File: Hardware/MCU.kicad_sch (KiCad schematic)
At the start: 23 parts, among them U1 STM32F407VET6, U3 LAN8742A, Y1 25MHz

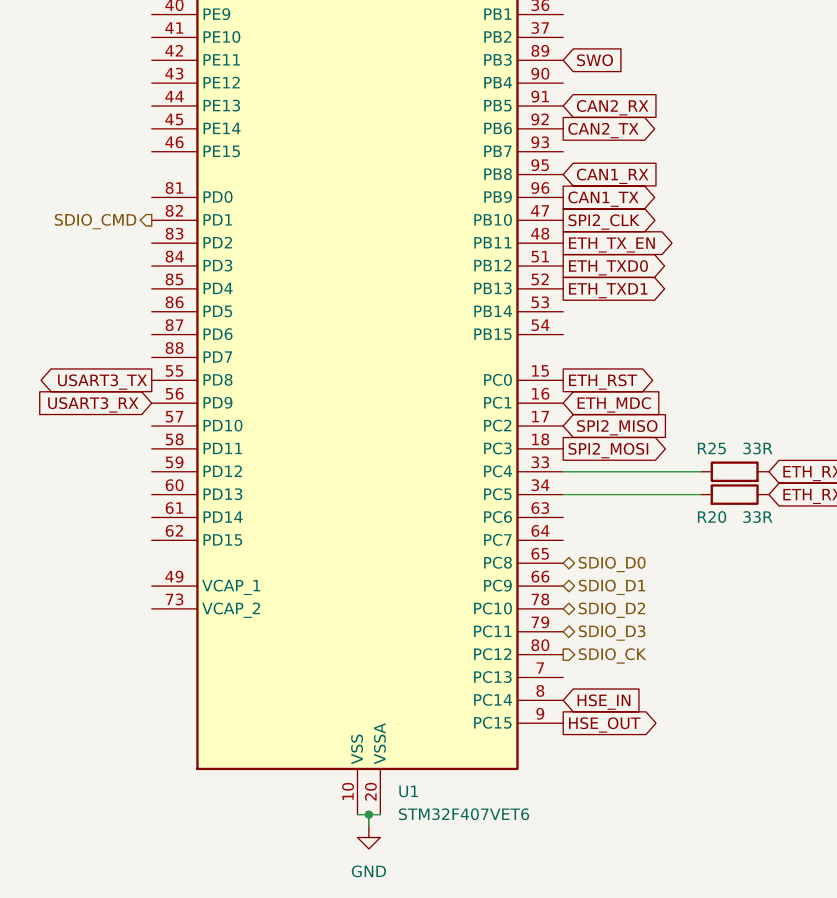
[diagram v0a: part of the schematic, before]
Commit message: added stepfiles
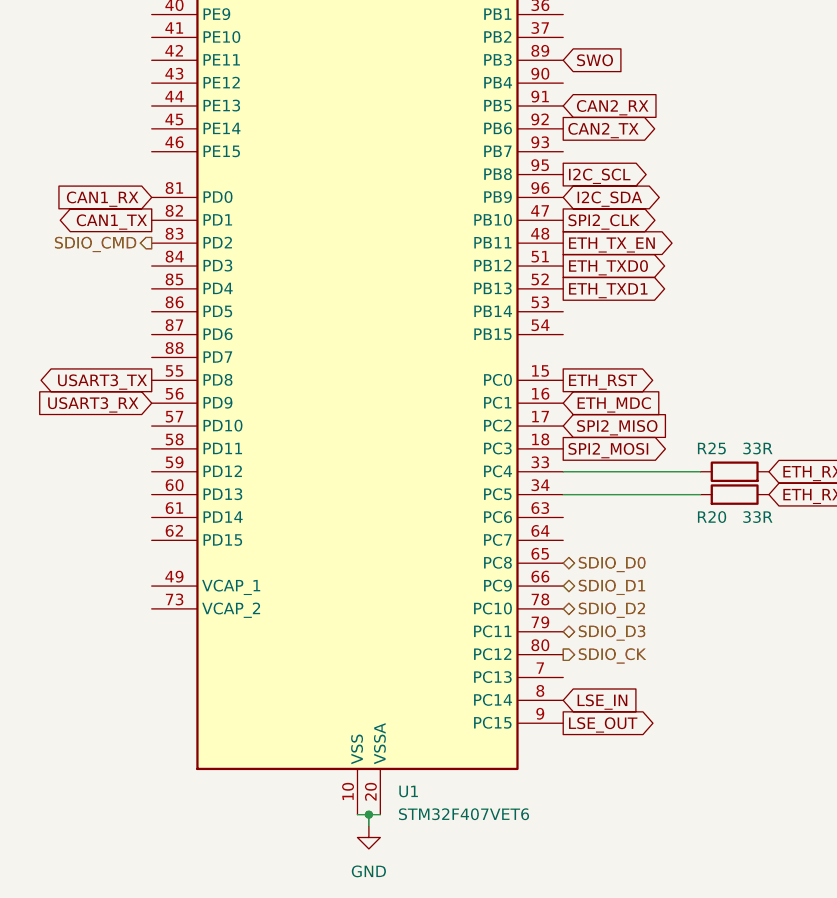
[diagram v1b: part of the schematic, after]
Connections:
- net CAN1_RX: now also U1.81 (PD0); no longer U1.95 (PB8)
- net CAN1_TX: now also U1.82 (PD1); no longer U1.96 (PB9)
- net HSE_IN: no longer U1.8 (PC14)
- net HSE_OUT: no longer U1.9 (PC15)
- net SDIO_CMD: now also U1.83 (PD2); no longer U1.82 (PD1)
- new net I2C_SCL: U1.95 (PB8)
- new net I2C_SDA: U1.96 (PB9)
- new net LSE_IN: U1.8 (PC14)
- new net LSE_OUT: U1.9 (PC15)
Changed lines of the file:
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@@
+    )
+  )
+  (global_label "CAN1_RX" (shape input) (at 41.91 106.68 180) (fields_autoplaced)
+    (effects (font (size 1.27 1.27)) (justify right))
+    (property "Intersheetrefs" "${INTERSHEET_REFS}" (at 30.6585 106.68 0)
+      (effects (font (size 1.27 1.27)) (justify right) hide)
     )
   )
@@
     )
   )
-  (global_label "HSE_OUT" (shape output) (at 87.63 165.1 0) (fields_autoplaced)
-    (effects (font (size 1.27 1.27)) (justify left))
-    (property "Intersheetrefs" "${INTERSHEET_REFS}" (at 98.821 165.1 0)
-      (effects (font (size 1.27 1.27)) (justify left) hide)
-    )
-  )
-  (global_label "CAN1_TX" (shape output) (at 87.63 106.68 0) (fields_autoplaced)
-    (effects (font (size 1.27 1.27)) (justify left))
-    (property "Intersheetrefs" "${INTERSHEET_REFS}" (at 98.5791 106.68 0)
+  (global_label "LSE_OUT" (shape output) (at 87.63 165.1 0) (fields_autoplaced)
+    (effects (font (size 1.27 1.27)) (justify left))
+    (property "Intersheetrefs" "${INTERSHEET_REFS}" (at 98.5186 165.1 0)
       (effects (font (size 1.27 1.27)) (justify left) hide)
     )
@@
     )
   )
-  (global_label "CAN1_RX" (shape input) (at 87.63 104.14 0) (fields_autoplaced)
-    (effects (font (size 1.27 1.27)) (justify left))
-    (property "Intersheetrefs" "${INTERSHEET_REFS}" (at 98.8815 104.14 0)
-      (effects (font (size 1.27 1.27)) (justify left) hide)
-    )
-  )
   (global_label "USART3_RX" (shape input) (at 41.91 129.54 180) (fields_autoplaced)
     (effects (font (size 1.27 1.27)) (justify right))
@@
     )
   )
+  (global_label "I2C_SDA" (shape bidirectional) (at 87.63 106.68 0) (fields_autoplaced)
+    (effects (font (size 1.27 1.27)) (justify left))
+    (property "Intersheetrefs" "${INTERSHEET_REFS}" (at 99.2671 106.68 0)
+      (effects (font (size 1.27 1.27)) (justify left) hide)
+    )
+  )
   (global_label "ETH_MDC" (shape output) (at 195.58 129.54 180) (fields_autoplaced)
     (effects (font (size 1.27 1.27)) (justify right))
@@
     )
   )
+  (global_label "CAN1_TX" (shape output) (at 41.91 109.22 180) (fields_autoplaced)
+    (effects (font (size 1.27 1.27)) (justify right))
+    (property "Intersheetrefs" "${INTERSHEET_REFS}" (at 30.9609 109.22 0)
+      (effects (font (size 1.27 1.27)) (justify right) hide)
+    )
+  )
+  (global_label "I2C_SCL" (shape output) (at 87.63 104.14 0) (fields_autoplaced)
+    (effects (font (size 1.27 1.27)) (justify left))
+    (property "Intersheetrefs" "${INTERSHEET_REFS}" (at 98.0953 104.14 0)
+      (effects (font (size 1.27 1.27)) (justify left) hide)
+    )
+  )
   (global_label "ETH_TXD1" (shape input) (at 195.58 111.76 180) (fields_autoplaced)
     (effects (font (size 1.27 1.27)) (justify right))
@@
     )
   )
-  (global_label "HSE_IN" (shape input) (at 87.63 162.56 0) (fields_autoplaced)
-    (effects (font (size 1.27 1.27)) (justify left))
-    (property "Intersheetrefs" "${INTERSHEET_REFS}" (at 97.1277 162.56 0)
+  (global_label "LSE_IN" (shape input) (at 87.63 162.56 0) (fields_autoplaced)
+    (effects (font (size 1.27 1.27)) (justify left))
+    (property "Intersheetrefs" "${INTERSHEET_REFS}" (at 96.8253 162.56 0)
       (effects (font (size 1.27 1.27)) (justify left) hide)
     )
@@
     (effects (font (size 1.27 1.27)) (justify left))
   )
-  (hierarchical_label "SDIO_CMD" (shape output) (at 41.91 109.22 180) (fields_autoplaced)
-    (effects (font (size 1.27 1.27)) (justify right))
-  )
   (hierarchical_label "SDIO_D2" (shape bidirectional) (at 87.63 152.4 0) (fields_autoplaced)
     (effects (font (size 1.27 1.27)) (justify left))
@@
     (effects (font (size 1.27 1.27)) (justify left))
   )
+  (hierarchical_label "SDIO_CMD" (shape output) (at 41.91 111.76 180) (fields_autoplaced)
+    (effects (font (size 1.27 1.27)) (justify right))
+  )
   (symbol (lib_id "Device:C") (at 190.5 153.67 0) (unit 1)
